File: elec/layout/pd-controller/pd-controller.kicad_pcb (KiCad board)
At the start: 2 copper layers, 26.4 x 17.6 mm, 19 parts, among them CN1 STEMMA_RIGHT_ANGLE, Q1 MOSFET, U1 STUSB4500QTR, U2 XT30PW

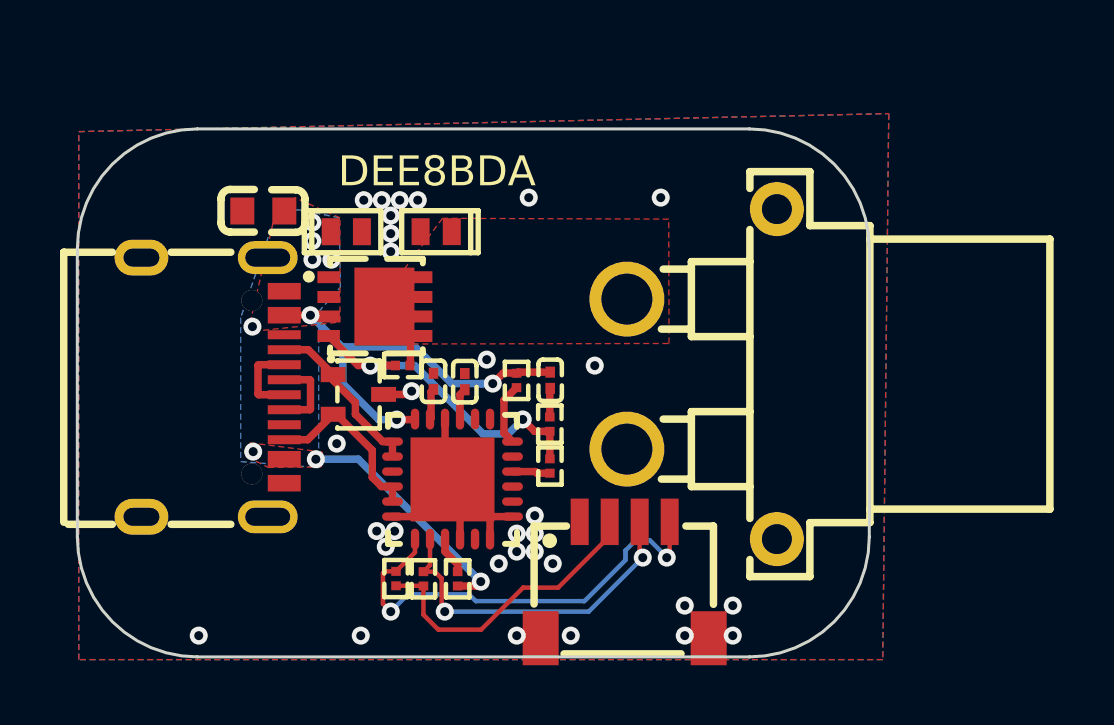
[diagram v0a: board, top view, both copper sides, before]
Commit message: update layout
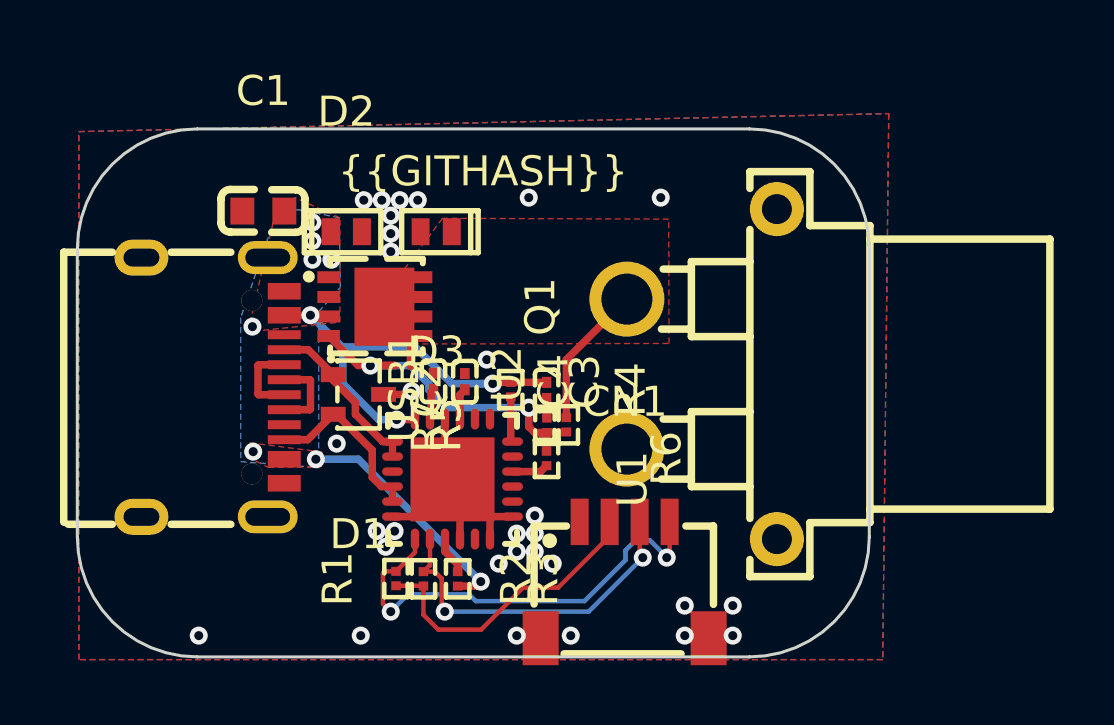
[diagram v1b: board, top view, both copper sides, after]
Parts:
- removed R8: 22.1kΩ ±1% 50mW, lcsc:R0201
- removed R9: 100Ω ±1% 50mW, lcsc:R0201
- added R4: 1kΩ ±1% 50mW, lcsc:R0201, F.Cu at (143.8, 97.8)
- added R5: 100kΩ ±1% 50mW, lcsc:R0201, F.Cu at (145.7, 99.0)
- R6: value 1kΩ ±1% 50mW -> 22.1kΩ ±1% 50mW
- R7: value 100kΩ ±1% 50mW -> 100Ω ±1% 50mW
- moved R7 5.20 mm to (145.0, 99.0), turned to 90 degrees
- moved R6 2.79 mm to (145.0, 100.1)
- moved C2 0.36 mm to (145.0, 97.8)
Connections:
- C2 pad 1: C2-1-R9-2 -> C2-1-R7-2
- Q1 pad 4: Q1-4-R7-1-R8-1-R9-1 -> Q1-4-R5-1-R6-1-R7-1
- R6 pad 1: VBUS -> Q1-4-R5-1-R6-1-R7-1
- R6 pad 2: R6-2-U1-18 -> R6-2-U1-16
- R7 pad 1: Q1-4-R7-1-R8-1-R9-1 -> Q1-4-R5-1-R6-1-R7-1
- R7 pad 2: VSINK_VCC -> C2-1-R7-2
- U1 pad 16: R8-2-U1-16 -> R6-2-U1-16
- U1 pad 18: R6-2-U1-18 -> R4-2-U1-18
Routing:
- net Q1-4-R5-1-R6-1-R7-1: track 0.00 -> 12.1 mm, vias 0 -> 2
- net Q1-4-R7-1-R8-1-R9-1: track 11.7 -> 0.00 mm, vias 2 -> 0
- net VSINK_VCC: track 2.35 -> 7.14 mm
- net R6-2-U1-18: track 2.09 -> 0.00 mm
- net R4-2-U1-18: track 0.00 -> 1.52 mm
- net R8-2-U1-16: track 1.27 -> 0.00 mm
- net R6-2-U1-16: track 0.00 -> 1.22 mm
- net C2-1-R9-2: track 0.96 -> 0.00 mm
- net C2-1-R7-2: track 0.00 -> 0.66 mm
- net GND: vias 31 -> 30
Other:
- board text added: "{{GITHASH}}"
- board text removed: "DEE8BDA"
